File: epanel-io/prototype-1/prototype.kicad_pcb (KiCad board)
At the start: 2 copper layers, 28 parts, among them J1 Conn_01x05_Male, J2 Screw_Terminal_01x02, J3 Screw_Terminal_01x02, J4 Screw_Terminal_01x02, Q1 IRF830, Q2 BT136-600, U1 4N35, U2 H11AA1, U3 MOC3021M

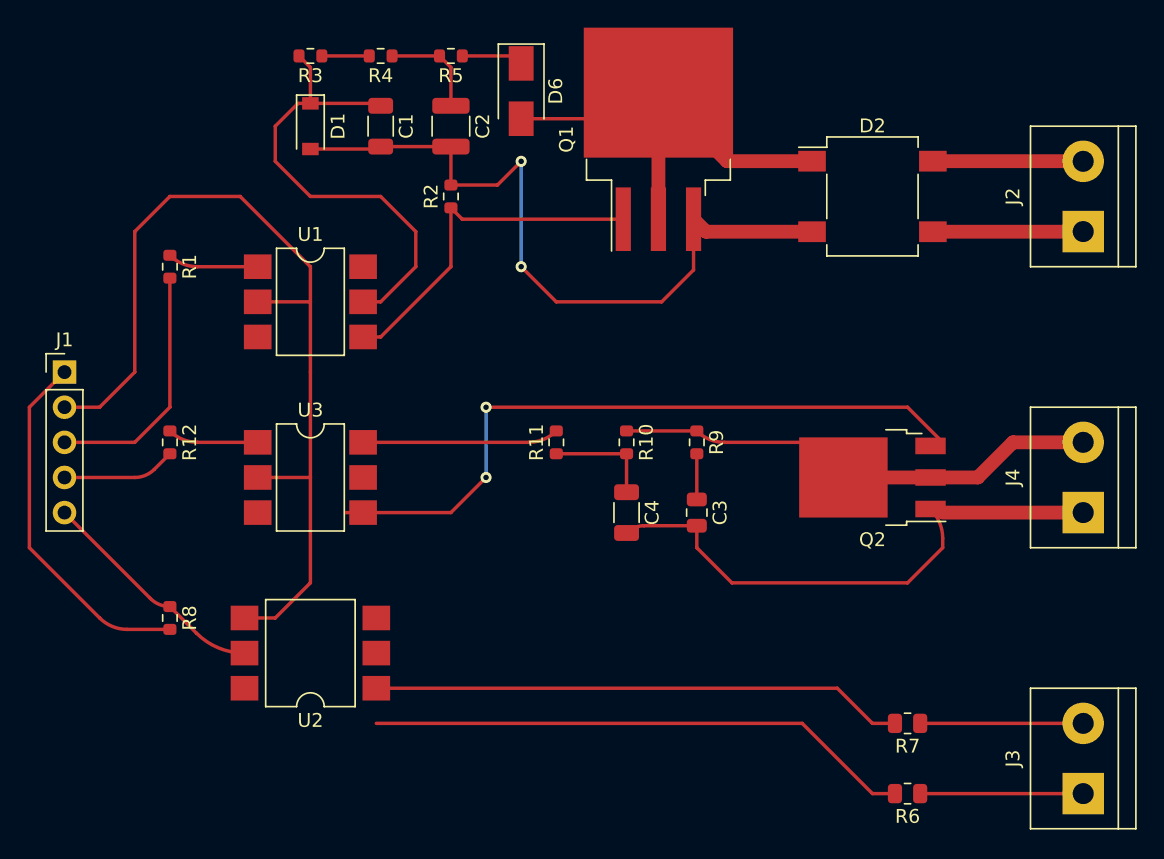
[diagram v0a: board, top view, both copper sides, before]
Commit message: fixes
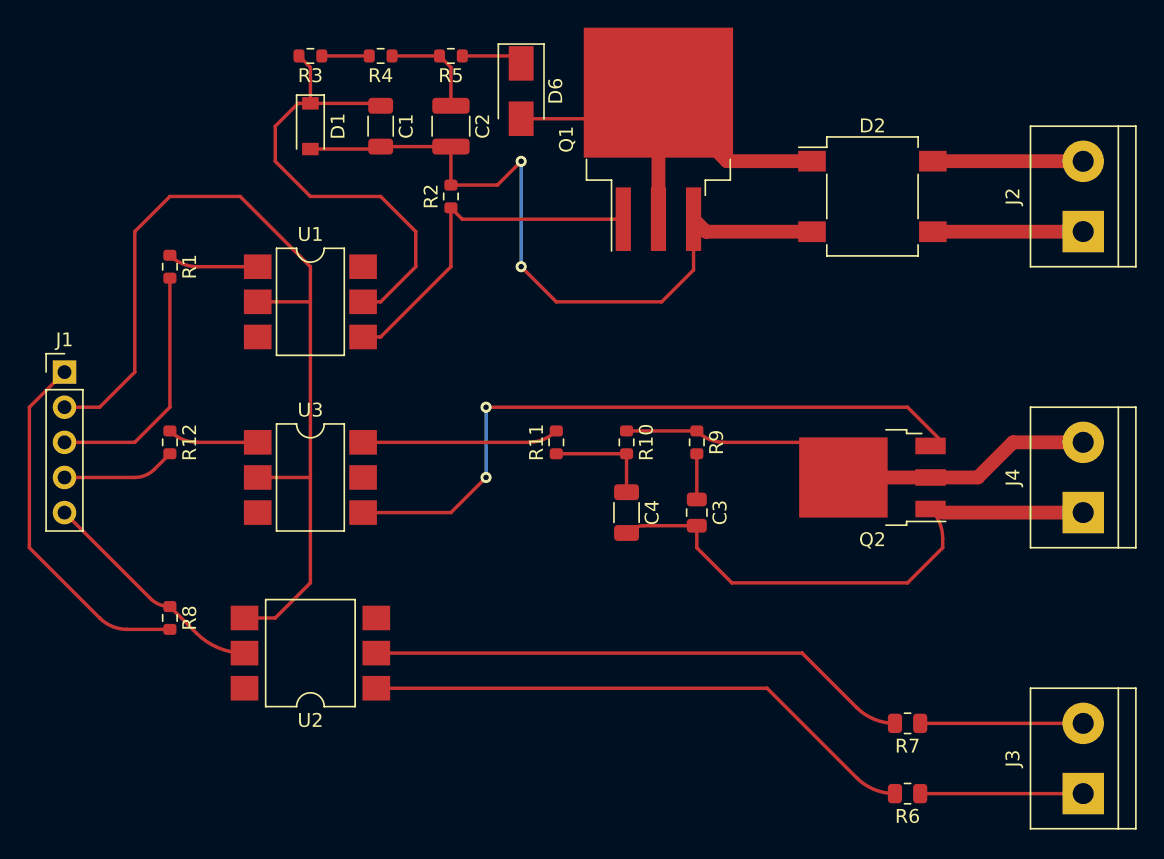
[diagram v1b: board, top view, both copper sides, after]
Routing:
- net Net-(Q2-Pad3): track 51.3 -> 50.0 mm
- net Net-(R7-Pad2): track 38.6 -> 39.4 mm
- net Net-(R6-Pad2): track 39.6 -> 40.5 mm
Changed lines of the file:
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@@
   (segment (start 101.6 71.12) (end 99.06 73.66) (width 0.25) (layer "F.Cu") (net 9))
   (arc (start 104.14 88.9) (mid 105.053811 89.51059) (end 106.131726 89.725) (width 0.25) (layer "F.Cu") (net 9))
-  (segment (start 119.38 78.74) (end 119.38 71.12) (width 0.25) (layer "F.Cu") (net 10))
   (segment (start 104.14 73.66) (end 101.6 73.66) (width 0.25) (layer "F.Cu") (net 10))
-  (segment (start 115.57 78.74) (end 116.84 78.74) (width 0.25) (layer "F.Cu") (net 10))
+  (segment (start 115.57 78.74) (end 119.38 78.74) (width 0.25) (layer "F.Cu") (net 10))
   (segment (start 119.38 63.5) (end 114.3 58.42) (width 0.25) (layer "F.Cu") (net 10))
   (segment (start 115.57 66.04) (end 119.38 66.04) (width 0.25) (layer "F.Cu") (net 10))
@@
   (segment (start 114.615 88.9) (end 116.84 88.9) (width 0.25) (layer "F.Cu") (net 10))
   (segment (start 114.3 58.42) (end 109.22 58.42) (width 0.25) (layer "F.Cu") (net 10))
-  (segment (start 116.84 78.74) (end 119.38 78.74) (width 0.25) (layer "F.Cu") (net 10))
   (segment (start 119.38 66.04) (end 119.38 63.5) (width 0.25) (layer "F.Cu") (net 10))
-  (segment (start 119.38 66.04) (end 119.38 71.12) (width 0.25) (layer "F.Cu") (net 10))
+  (segment (start 119.38 66.04) (end 119.38 78.74) (width 0.25) (layer "F.Cu") (net 10))
   (segment (start 119.38 86.36) (end 119.38 78.74) (width 0.25) (layer "F.Cu") (net 10))
   (segment (start 109.22 58.42) (end 106.68 60.96) (width 0.25) (layer "F.Cu") (net 10))
@@
   (segment (start 132.08 78.74) (end 129.54 81.28) (width 0.25) (layer "F.Cu") (net 17))
   (segment (start 164.472305 76.46) (end 164.22 76.46) (width 0.25) (layer "F.Cu") (net 17))
-  (segment (start 123.19 81.28) (end 121.92 81.28) (width 0.25) (layer "F.Cu") (net 17))
   (segment (start 162.56 73.66) (end 132.08 73.66) (width 0.25) (layer "F.Cu") (net 17))
   (segment (start 129.54 81.28) (end 123.19 81.28) (width 0.25) (layer "F.Cu") (net 17))
@@
   (arc (start 111.211726 63.5) (mid 110.133812 63.28559) (end 109.22 62.675) (width 0.25) (layer "F.Cu") (net 18))
   (segment (start 120.205 48.26) (end 123.635 48.26) (width 0.25) (layer "F.Cu") (net 19))
-  (segment (start 160.02 101.6) (end 154.94 96.52) (width 0.25) (layer "F.Cu") (net 20))
-  (segment (start 161.6475 101.6) (end 160.02 101.6) (width 0.25) (layer "F.Cu") (net 20))
-  (segment (start 154.94 96.52) (end 124.145 96.52) (width 0.25) (layer "F.Cu") (net 20))
-  (segment (start 161.6475 96.52) (end 160.02 96.52) (width 0.25) (layer "F.Cu") (net 21))
-  (segment (start 157.48 93.98) (end 124.145 93.98) (width 0.25) (layer "F.Cu") (net 21))
-  (segment (start 160.02 96.52) (end 157.48 93.98) (width 0.25) (layer "F.Cu") (net 21))
+  (segment (start 152.4 93.98) (end 158.869183 100.449184) (width 0.25) (layer "F.Cu") (net 20))
+  (segment (start 152.4 93.98) (end 124.145 93.98) (width 0.25) (layer "F.Cu") (net 20))
+  (arc (start 161.6475 101.6) (mid 160.143886 101.300913) (end 158.869183 100.449184) (width 0.25) (layer "F.Cu") (net 20))
+  (segment (start 158.869183 95.369184) (end 154.94 91.44) (width 0.25) (layer "F.Cu") (net 21))
+  (segment (start 154.94 91.44) (end 124.145 91.44) (width 0.25) (layer "F.Cu") (net 21))
+  (arc (start 161.6475 96.52) (mid 160.143886 96.220913) (end 158.869183 95.369184) (width 0.25) (layer "F.Cu") (net 21))
   (segment (start 135.168274 76.2) (end 123.19 76.2) (width 0.25) (layer "F.Cu") (net 22))
   (arc (start 137.16 75.375) (mid 136.246188 75.985589) (end 135.168274 76.2) (width 0.25) (layer "F.Cu") (net 22))
@@
   (segment (start 175.25 60.97) (end 175.26 60.96) (width 0.25) (layer "F.Cu") (net 30))
   (segment (start 164.39 60.97) (end 175.25 60.97) (width 1) (layer "F.Cu") (net 30))
-  (segment (start 164.4 60.96) (end 164.39 60.97) (width 0.25) (layer "F.Cu") (net 30))
   (segment (start 175.25 55.87) (end 175.26 55.88) (width 0.25) (layer "F.Cu") (net 31))
-  (segment (start 164.4 55.88) (end 164.39 55.87) (width 0.25) (layer "F.Cu") (net 31))
   (segment (start 164.39 55.87) (end 175.25 55.87) (width 1) (layer "F.Cu") (net 31))
   (segment (start 164.22 78.74) (end 167.64 78.74) (width 1) (layer "F.Cu") (net 32))
